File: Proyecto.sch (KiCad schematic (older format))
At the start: 54 parts, among them P1 CONN_01X03, P2 CONN_01X03, Q1 BC808-40, Q2 BC808-40, U1 MCP2515, U2 MCP2551-I/SN, U3 AMS1117, U4 ACS712, U5 ACS712, U6 AMS1117

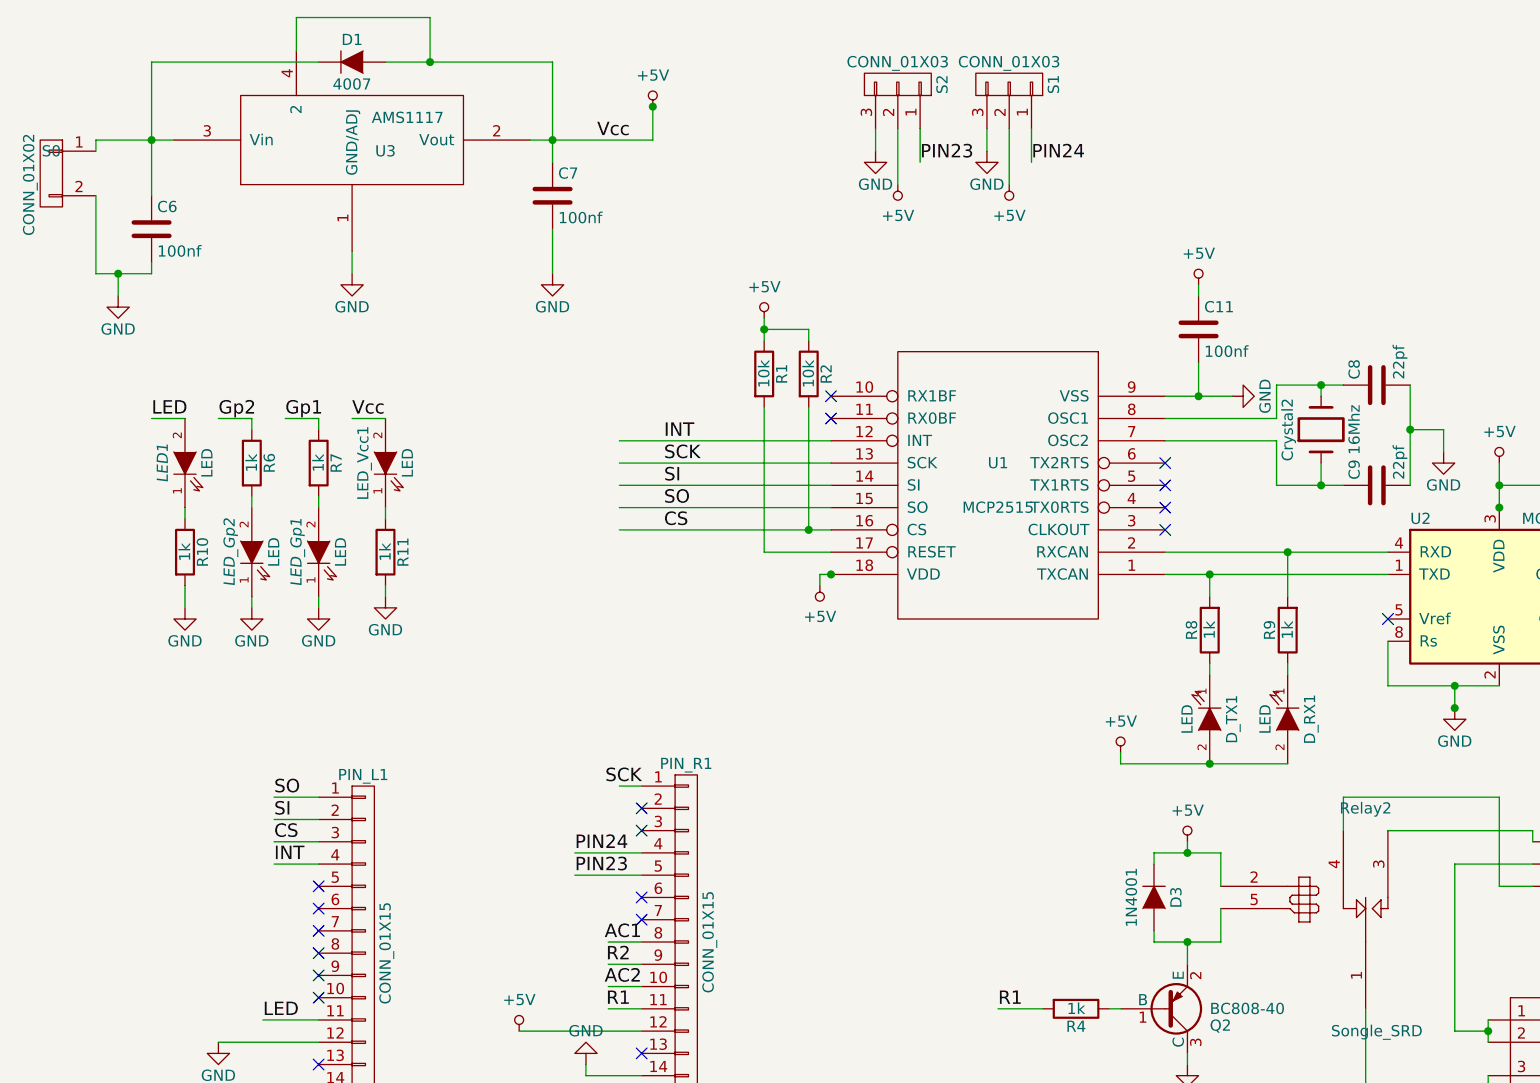
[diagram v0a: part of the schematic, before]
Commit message: casa
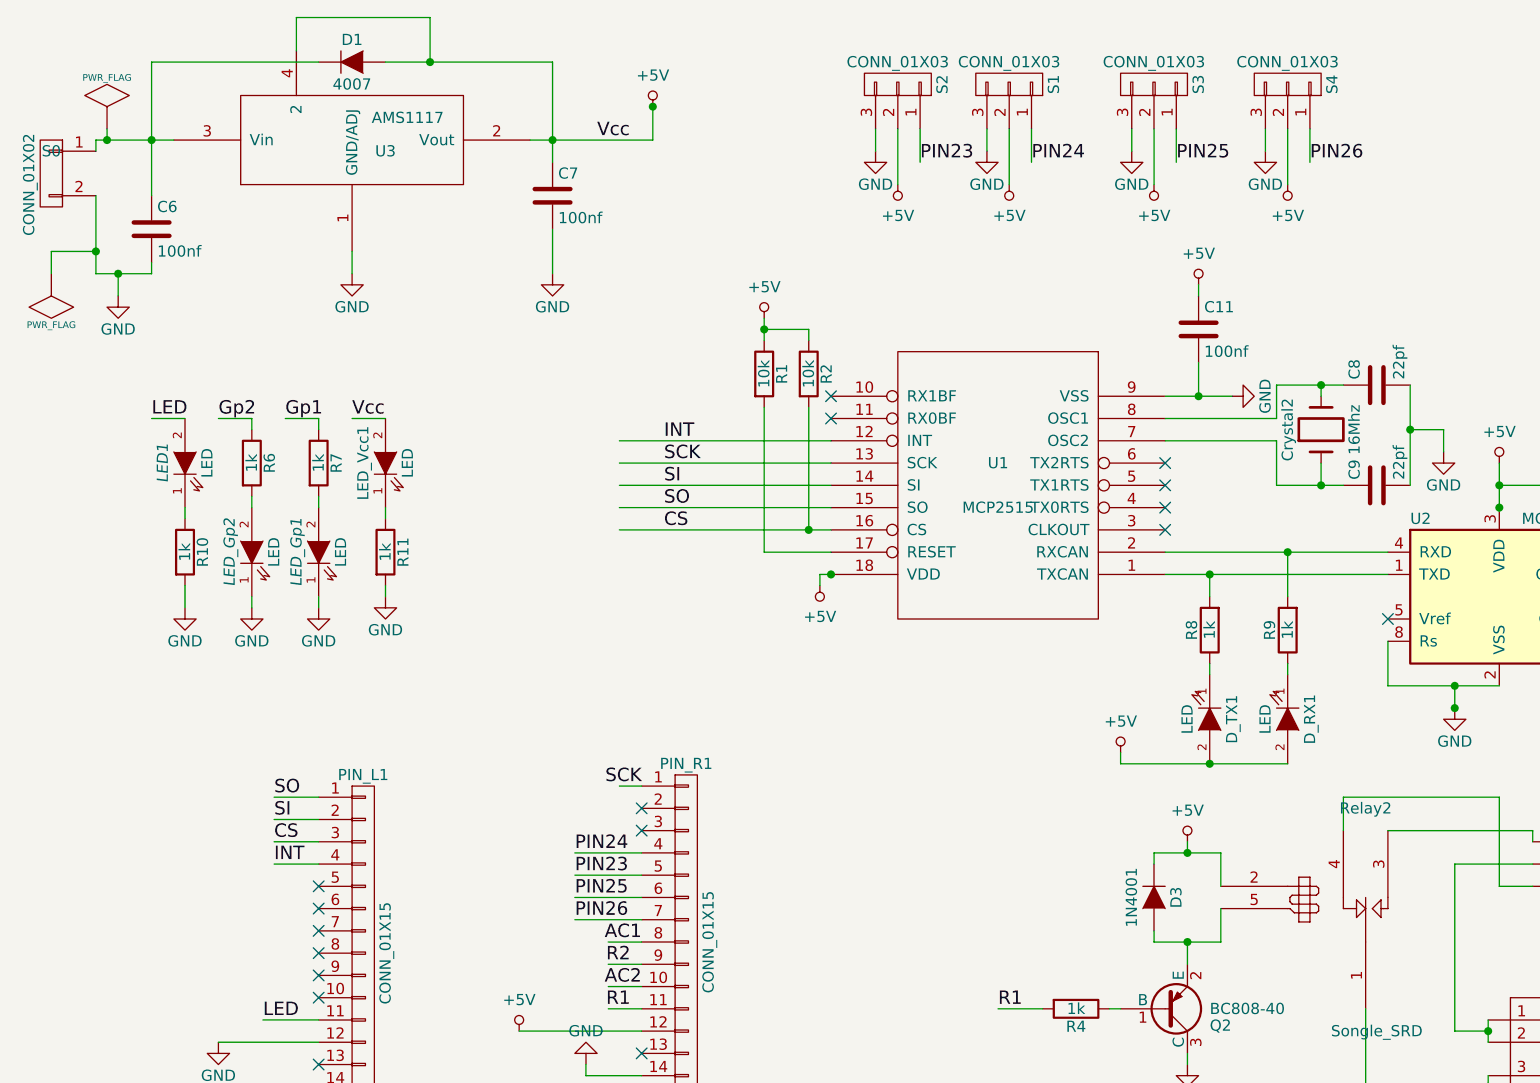
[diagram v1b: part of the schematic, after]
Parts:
- added S3, S4: CONN_01X03, Pin_Headers:Pin_Header_Straight_1x03, symbol CONN_01X03
- PIN_L1, PIN_R1: footprint w_pin_strip:pin_socket_2mm_15 -> w_pin_strip:pin_socket_15
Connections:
- net labels added: PIN25, PIN26
- wire segments 207 -> 218
- no-connect marks 22 -> 20
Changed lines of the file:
@@
 F 0 "PIN_R1" H 3550 5550 50  0000 C CNN
 F 1 "CONN_01X15" V 3650 4750 50  0000 C CNN
-F 2 "w_pin_strip:pin_socket_2mm_15" H 3550 4750 50  0001 C CNN
+F 2 "w_pin_strip:pin_socket_15" H 3550 4750 50  0001 C CNN
 F 3 "" H 3550 4750 50  0000 C CNN
 	1    3550 4750
@@
 F 0 "PIN_L1" H 2100 5600 50  0000 C CNN
 F 1 "CONN_01X15" V 2200 4800 50  0000 C CNN
-F 2 "w_pin_strip:pin_socket_2mm_15" H 2100 4800 50  0001 C CNN
+F 2 "w_pin_strip:pin_socket_15" H 2100 4800 50  0001 C CNN
 F 3 "" H 2100 4800 50  0000 C CNN
 	1    2100 4800
@@
 $EndComp
 NoConn ~ 3350 5250
-NoConn ~ 3350 4650
-NoConn ~ 3350 4550
 NoConn ~ 3350 4250
 Text Label 6150 6750 0    60   ~ 0
@@
 Connection ~ 1700 7250
 NoConn ~ 3350 4150
+$Comp
+L PWR_FLAG #FLG042
+U 1 1 57840DBD
+P 950 1100
+F 0 "#FLG042" H 950 1370 30  0001 C CNN
+F 1 "PWR_FLAG" H 950 1330 30  0000 C CNN
+F 2 "" H 950 1100 60  0000 C CNN
+F 3 "" H 950 1100 60  0000 C CNN
+	1    950  1100
+	1    0    0    -1
+$EndComp
+Wire Wire Line
+	950  1100 950  1150
+Connection ~ 950  1150
+$Comp
+L PWR_FLAG #FLG043
+U 1 1 57841CE9
+P 700 1750
+F 0 "#FLG043" H 700 2020 30  0001 C CNN
+F 1 "PWR_FLAG" H 700 1980 30  0000 C CNN
+F 2 "" H 700 1750 60  0000 C CNN
+F 3 "" H 700 1750 60  0000 C CNN
+	1    700  1750
+	-1   0    0    1
+$EndComp
+Wire Wire Line
+	700  1750 700  1650
+Wire Wire Line
+	700  1650 900  1650
+Connection ~ 900  1650
+$Comp
+L CONN_01X03 S3
+U 1 1 57841E7A
+P 5650 900
+F 0 "S3" H 5650 1100 50  0000 C CNN
+F 1 "CONN_01X03" V 5750 900 50  0000 C CNN
+F 2 "Pin_Headers:Pin_Header_Straight_1x03" H 5650 900 50  0001 C CNN
+F 3 "" H 5650 900 50  0000 C CNN
+	1    5650 900
+	0    1    -1   0
+$EndComp
+$Comp
+L +5V #PWR044
+U 1 1 57841E80
+P 5650 1350
+F 0 "#PWR044" H 5650 1200 50  0001 C CNN
+F 1 "+5V" H 5650 1490 50  0000 C CNN
+F 2 "" H 5650 1350 50  0000 C CNN
+F 3 "" H 5650 1350 50  0000 C CNN
+	1    5650 1350
+	-1   0    0    1
+$EndComp
+$Comp
+L GND-RESCUE-Proyecto #PWR045
+U 1 1 57841E86
+P 5550 1200
+F 0 "#PWR045" H 5550 950 50  0001 C CNN
+F 1 "GND" H 5550 1050 50  0000 C CNN
+F 2 "" H 5550 1200 50  0000 C CNN
+F 3 "" H 5550 1200 50  0000 C CNN
+	1    5550 1200
+	1    0    0    -1
+$EndComp
+Wire Wire Line
+	5550 1100 5550 1200
+Wire Wire Line
+	5650 1100 5650 1350
+Wire Wire Line
+	5750 1100 5750 1250
+Text Label 5750 1250 0    60   ~ 0
+PIN25
+$Comp
+L CONN_01X03 S4
+U 1 1 57841F1D
+P 6250 900
+F 0 "S4" H 6250 1100 50  0000 C CNN
+F 1 "CONN_01X03" V 6350 900 50  0000 C CNN
+F 2 "Pin_Headers:Pin_Header_Straight_1x03" H 6250 900 50  0001 C CNN
+F 3 "" H 6250 900 50  0000 C CNN
+	1    6250 900
+	0    1    -1   0
+$EndComp
+$Comp
+L +5V #PWR046
+U 1 1 57841F23
+P 6250 1350
+F 0 "#PWR046" H 6250 1200 50  0001 C CNN
+F 1 "+5V" H 6250 1490 50  0000 C CNN
+F 2 "" H 6250 1350 50  0000 C CNN
+F 3 "" H 6250 1350 50  0000 C CNN
+	1    6250 1350
+	-1   0    0    1
+$EndComp
+$Comp
+L GND-RESCUE-Proyecto #PWR047
+U 1 1 57841F29
+P 6150 1200
+F 0 "#PWR047" H 6150 950 50  0001 C CNN
+F 1 "GND" H 6150 1050 50  0000 C CNN
+F 2 "" H 6150 1200 50  0000 C CNN
+F 3 "" H 6150 1200 50  0000 C CNN
+	1    6150 1200
+	1    0    0    -1
+$EndComp
+Wire Wire Line
+	6150 1100 6150 1200
+Wire Wire Line
+	6250 1100 6250 1350
+Wire Wire Line
+	6350 1100 6350 1250
+Text Label 6350 1250 0    60   ~ 0
+PIN26
+Wire Wire Line
+	3350 4550 3050 4550
+Text Label 3050 4550 0    60   ~ 0
+PIN25
+Wire Wire Line
+	3350 4650 3050 4650
+Text Label 3050 4650 0    60   ~ 0
+PIN26
 $EndSCHEMATC
